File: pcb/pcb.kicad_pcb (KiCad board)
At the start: 2 copper layers, 100 x 80 mm, 20 parts, among them K1 Generic_Relay, K2 Generic_Relay, Q1 BC547, Q2 BC547

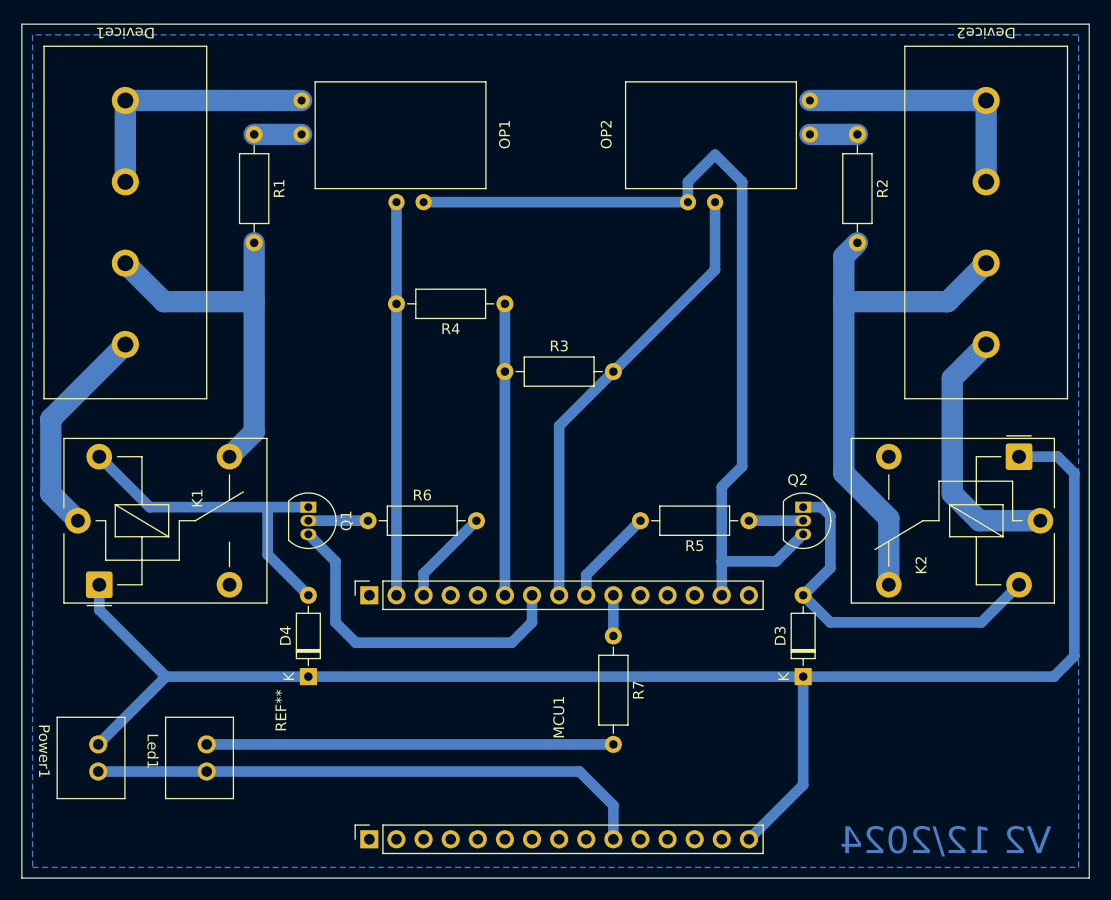
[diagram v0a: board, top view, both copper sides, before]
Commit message: Update optocoupler footprint and PCB with new model
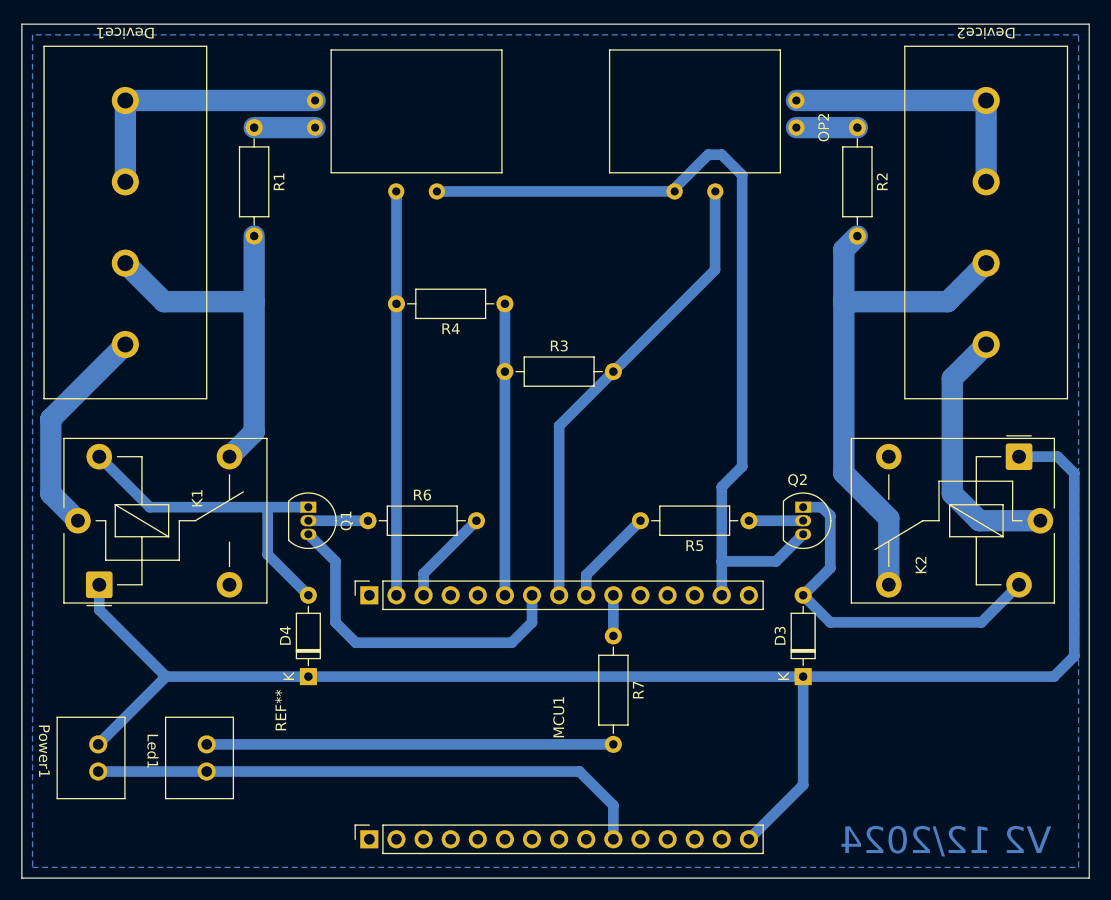
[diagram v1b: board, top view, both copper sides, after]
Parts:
- OP1: value Optocoupler_L -> Optocoupler_Left; footprint Custom_Footprints:Optocoupler_L -> Custom_Footprints:Optocoupler_Left
- OP2: value Optocoupler_R -> Optocoupler_Right; footprint Custom_Footprints:Optocoupler_R -> Custom_Footprints:Optocoupler_Right
- moved OP2 1.60 mm to (151.2, 65.7)
- moved OP1 1.60 mm to (128.9, 65.7)
- moved R1 0.64 mm to (111.8, 59.7)
- moved R2 0.64 mm to (168.3, 59.7)
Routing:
- net Net-(OP1-LDR1): track 82.8 -> 80.5 mm
- net Net-(OP2-IN1): track 4.44 -> 5.72 mm
- net Net-(Device2-Pin_1): track 24.1 -> 25.4 mm
- net Net-(OP1-IN1): track 4.44 -> 5.71 mm
- net Net-(Device1-Pin_1): track 24.1 -> 25.4 mm
- net Net-(MCU1-D5): track 42.9 -> 43.9 mm
- net Net-(MCU1-D1): track 36.8 -> 37.8 mm
- net Net-(Device2-Pin_3): track 49.1 -> 49.8 mm
- net Net-(Device1-Pin_3): track 34.6 -> 35.2 mm
